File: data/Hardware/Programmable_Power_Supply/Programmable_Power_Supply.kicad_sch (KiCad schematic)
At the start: 23 parts, among them J3 USB_C_Receptacle_USB2.0_14P, J4 Conn_01x05_Pin, J5 Conn_01x02_Pin, Q6 BSC050N03LS_G, SW1 SW_Push, SW2 SW_Push, U1 STM32G431CBT6, U6 USBLC6-2SC6

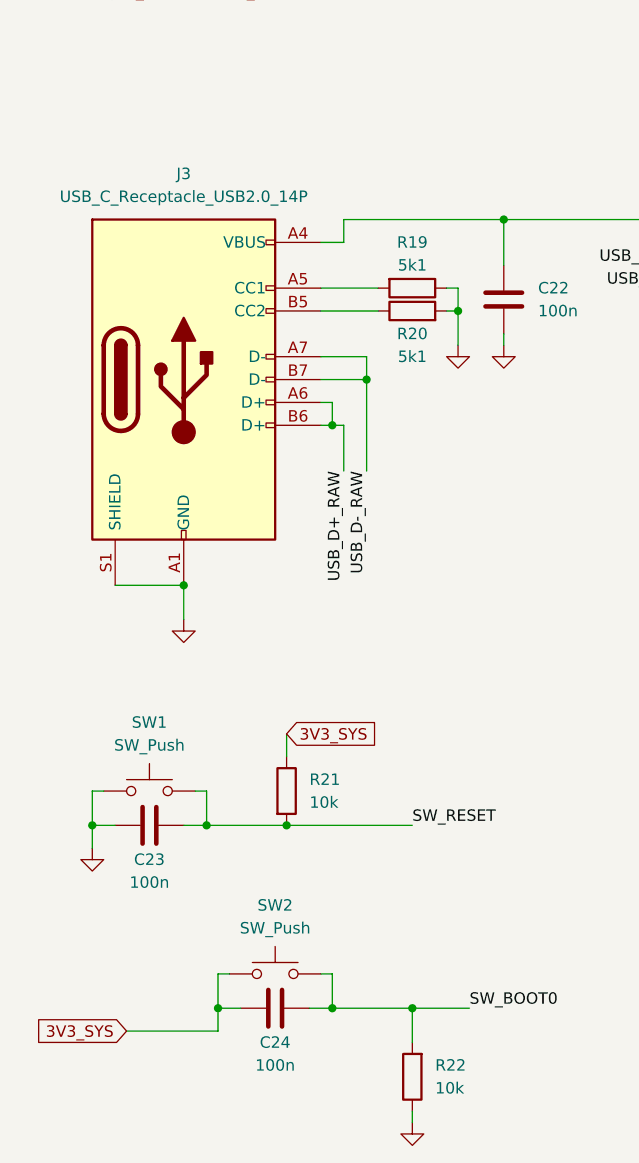
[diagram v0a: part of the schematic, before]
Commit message: feat: Final version of revision A of the schematic with mouser product numbers attached.
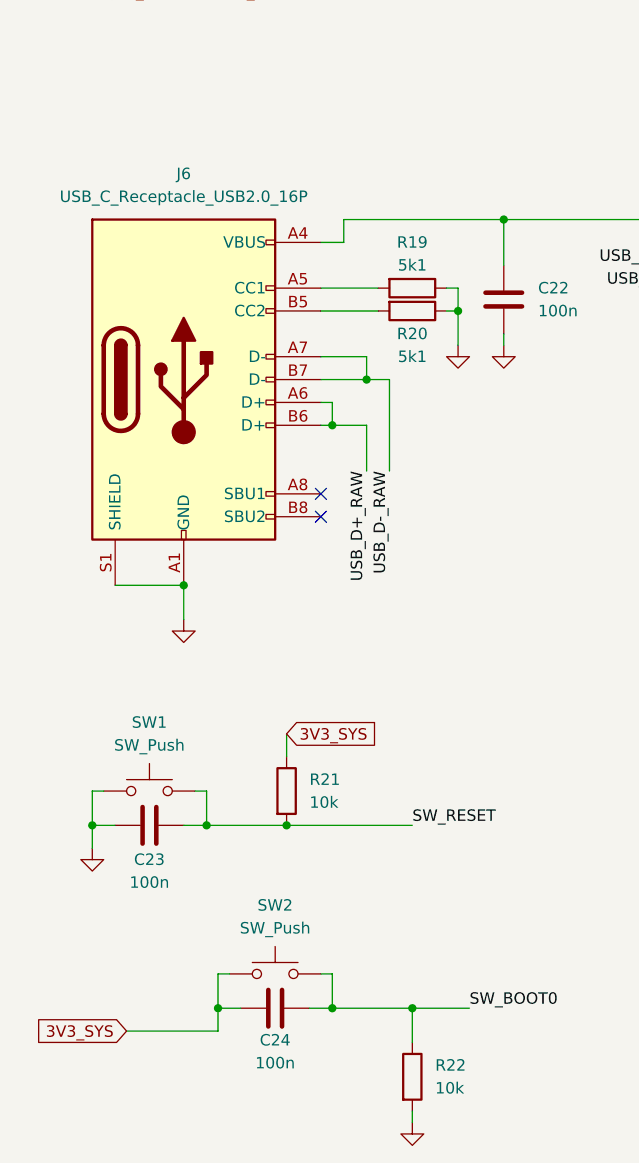
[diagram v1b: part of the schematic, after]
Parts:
- removed J3: USB_C_Receptacle_USB2.0_14P, Connector_USB:USB_C_Receptacle_HRO_TYPE-C-31-M-12, symbol Connector:USB_C_Receptacle_USB2.0_14P
- added J6: USB_C_Receptacle_USB2.0_16P, Connector_USB:USB_C_Receptacle_GCT_USB4105-xx-A_16P_TopMnt_Horizontal, symbol Connector:USB_C_Receptacle_USB2.0_16P
- C17, C18, C19, C20, C22, C23, C24: footprint Capacitor_SMD:C_0805_2012Metric_Pad1.18x1.45mm_HandSolder -> Capacitor_SMD:C_0201_0603Metric_Pad0.64x0.40mm_HandSolder; Mouser (none) -> MLASG063SB5104KFNA01
- C21: Mouser (none) -> GXT31CR6YA106KE01L
- D2: footprint Diode_THT:D_DO-35_SOD27_P7.62mm_Horizontal -> Szymon_Piorun_Library:SOD323; Mouser (none) -> 1N4148WS-HE3_A-18
- J4: now left out of the parts list
- J5: Mouser (none) -> 22-23-2021
- Q6: footprint Package_SON:Infineon_PG-TDSON-8_6.15x5.15mm -> Szymon_Piorun_Library:Infineon_PG-TDSON-8_6.15x5.15mm; Mouser (none) -> BSC030N03LS G
- R19, R20: Mouser (none) -> CR0603-FX-5101ELF
- R21, R22, R28: Mouser (none) -> RCA060310K0FKEC
- R27: Mouser (none) -> RT0603BRB07100RL
- SW1, SW2: footprint Button_Switch_SMD:SW_Push_1P1T_NO_CK_KSC6xxG -> Szymon_Piorun_Library:TS046650BK100SMTTR; Mouser (none) -> TS04-66-50-BK-100-SMT-TR
- U1: Mouser (none) -> STM32G431CBT6
- U6: Mouser (none) -> USBLC6-2SC6
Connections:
- net GND: now also C23.1, R20.1, R22.2, J6.A1 (GND), J6.A12 (GND), J6.B1 (GND), J6.B12 (GND), J6.S1 (SHIELD); no longer C23.2, R20.2, R22.1
- net SW_BOOT0: now also R22.1; no longer R22.2
- net SW_RESET: now also C23.2; no longer C23.1
- net USB_D+_RAW: now also J6.A6 (D+), J6.B6 (D+)
- net USB_D-_RAW: now also J6.A7 (D-), J6.B7 (D-)
- net at C22.1, U6.5 (VBUS): now also J6.A4 (VBUS), J6.A9 (VBUS), J6.B4 (VBUS), J6.B9 (VBUS)
- net at R19.2: now also J6.A5 (CC1)
- new net: J6.B5 (CC2), R20.2
- no-connect marks 25 -> 27

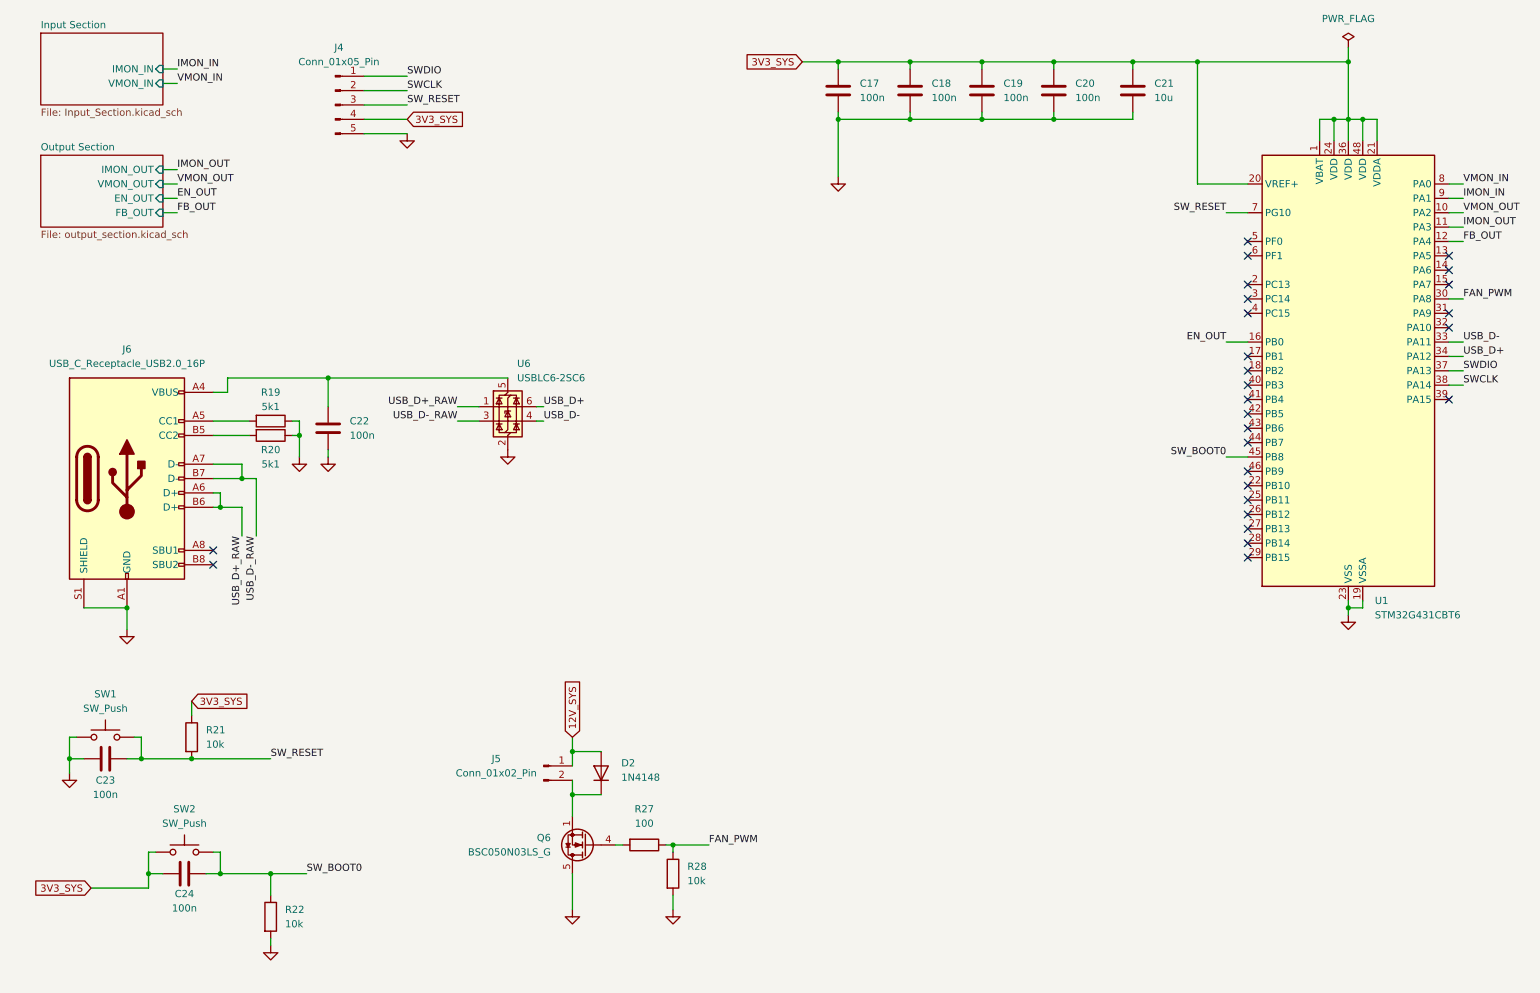
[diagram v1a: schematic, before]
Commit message: feat: First full layout of the PCB
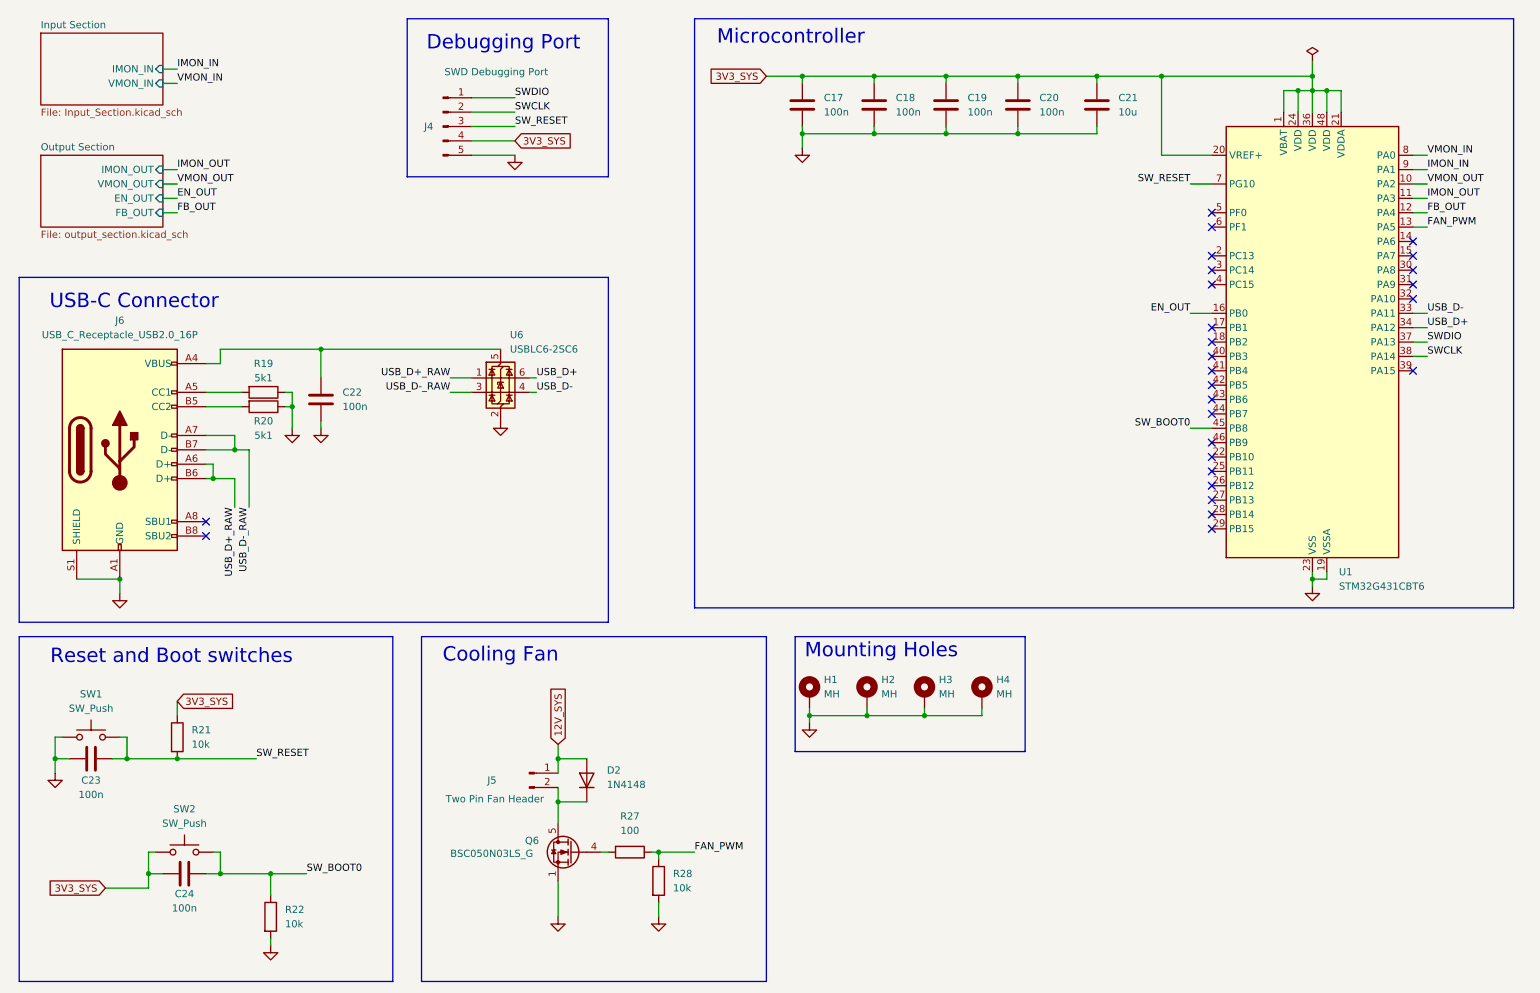
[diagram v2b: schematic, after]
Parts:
- added H1, H2, H3, H4: MH, MountingHole:MountingHole_3.2mm_M3_ISO7380_Pad_TopBottom, symbol Mechanical:MountingHole_Pad
- J4: value Conn_01x05_Pin -> SWD Debugging Port
- J5: value Conn_01x02_Pin -> Two Pin Fan Header
- Q6: Mouser BSC030N03LS G -> (none)
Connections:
- net FAN_PWM: now also U1.13 (PA5); no longer U1.30 (PA8)
- net GND: now also Q6.1 (S), Q6.2 (S), Q6.3 (S), H1.1, H2.1, H3.1, H4.1; no longer Q6.5 (D), Q6.6 (D), Q6.7 (D), Q6.8 (D)
- new net: D2.1 (K), J5.2 (Pin_2), Q6.5 (D)
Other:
- note added: "Cooling Fan"
- note added: "Debugging Port"
- note added: "Microcontroller"
- note added: "Mounting Holes"
- note added: "Reset and Boot switches"
- note added: "USB-C Connector"
- moved on the sheet: C17, C18, C19, C20, C21, C22, C23, D2, J4, J5, J6, R19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
